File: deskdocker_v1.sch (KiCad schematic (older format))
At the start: 117 parts, among them J1 USB_C_Receptacle_USB2.0, J2 USB_C_Receptacle_USB2.0, J3 OLED, SW1 SW_PUSH, SW10 SW_PUSH, SW11 SW_PUSH, SW12 SW_PUSH, SW13 SW_PUSH, SW14 SW_PUSH, SW15 SW_PUSH, SW16 SW_PUSH, SW17 SW_PUSH, SW18 SW_PUSH, SW19 Rotary_Encoder, SW2 SW_PUSH, SW20 SW_PUSH, SW21 SW_PUSH, SW22 SW_PUSH, SW23 SW_PUSH, SW24 SW_PUSH, SW3 SW_PUSH, SW4 SW_PUSH, SW5 SW_PUSH, SW6 SW_PUSH, SW7 SW_PUSH, SW8 SW_PUSH, SW9 SW_PUSH, U1 ATMEGA32U4, U2 MIC5219-5.0YMM, X1 16Mhz

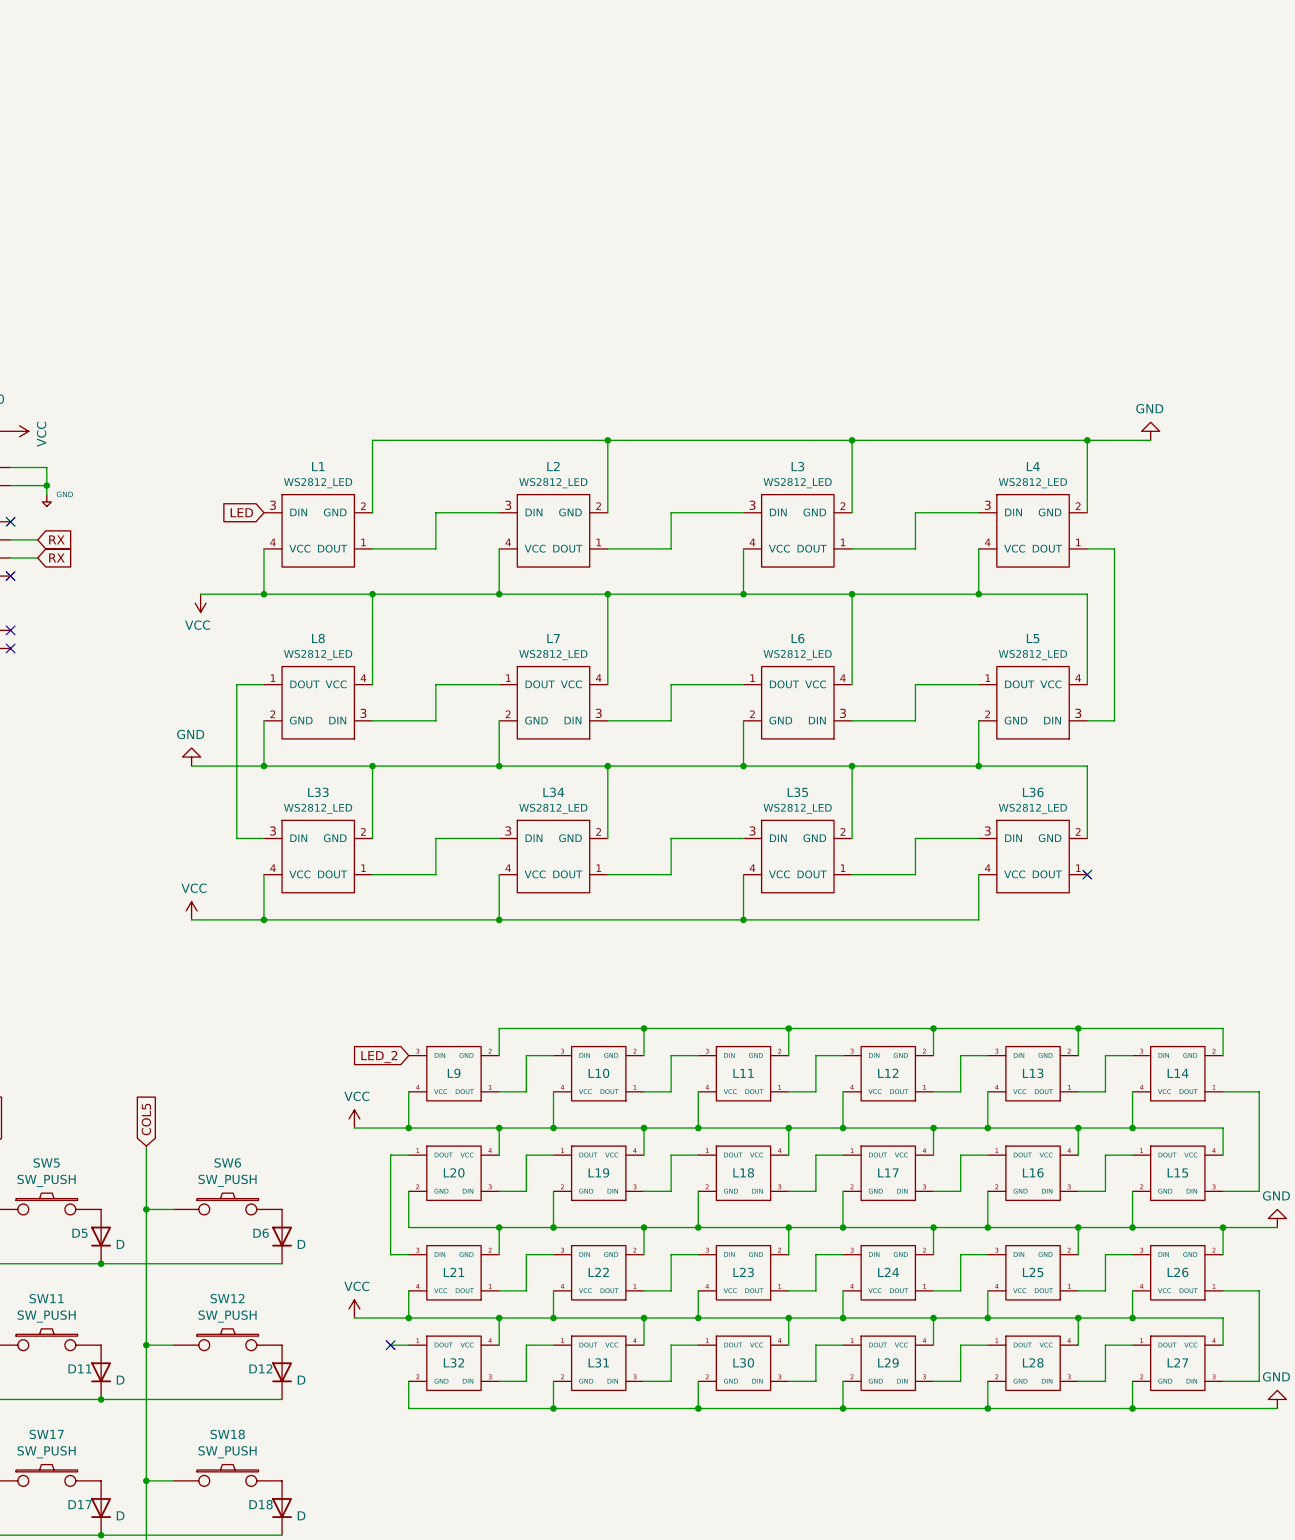
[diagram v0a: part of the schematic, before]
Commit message: schematic final_4
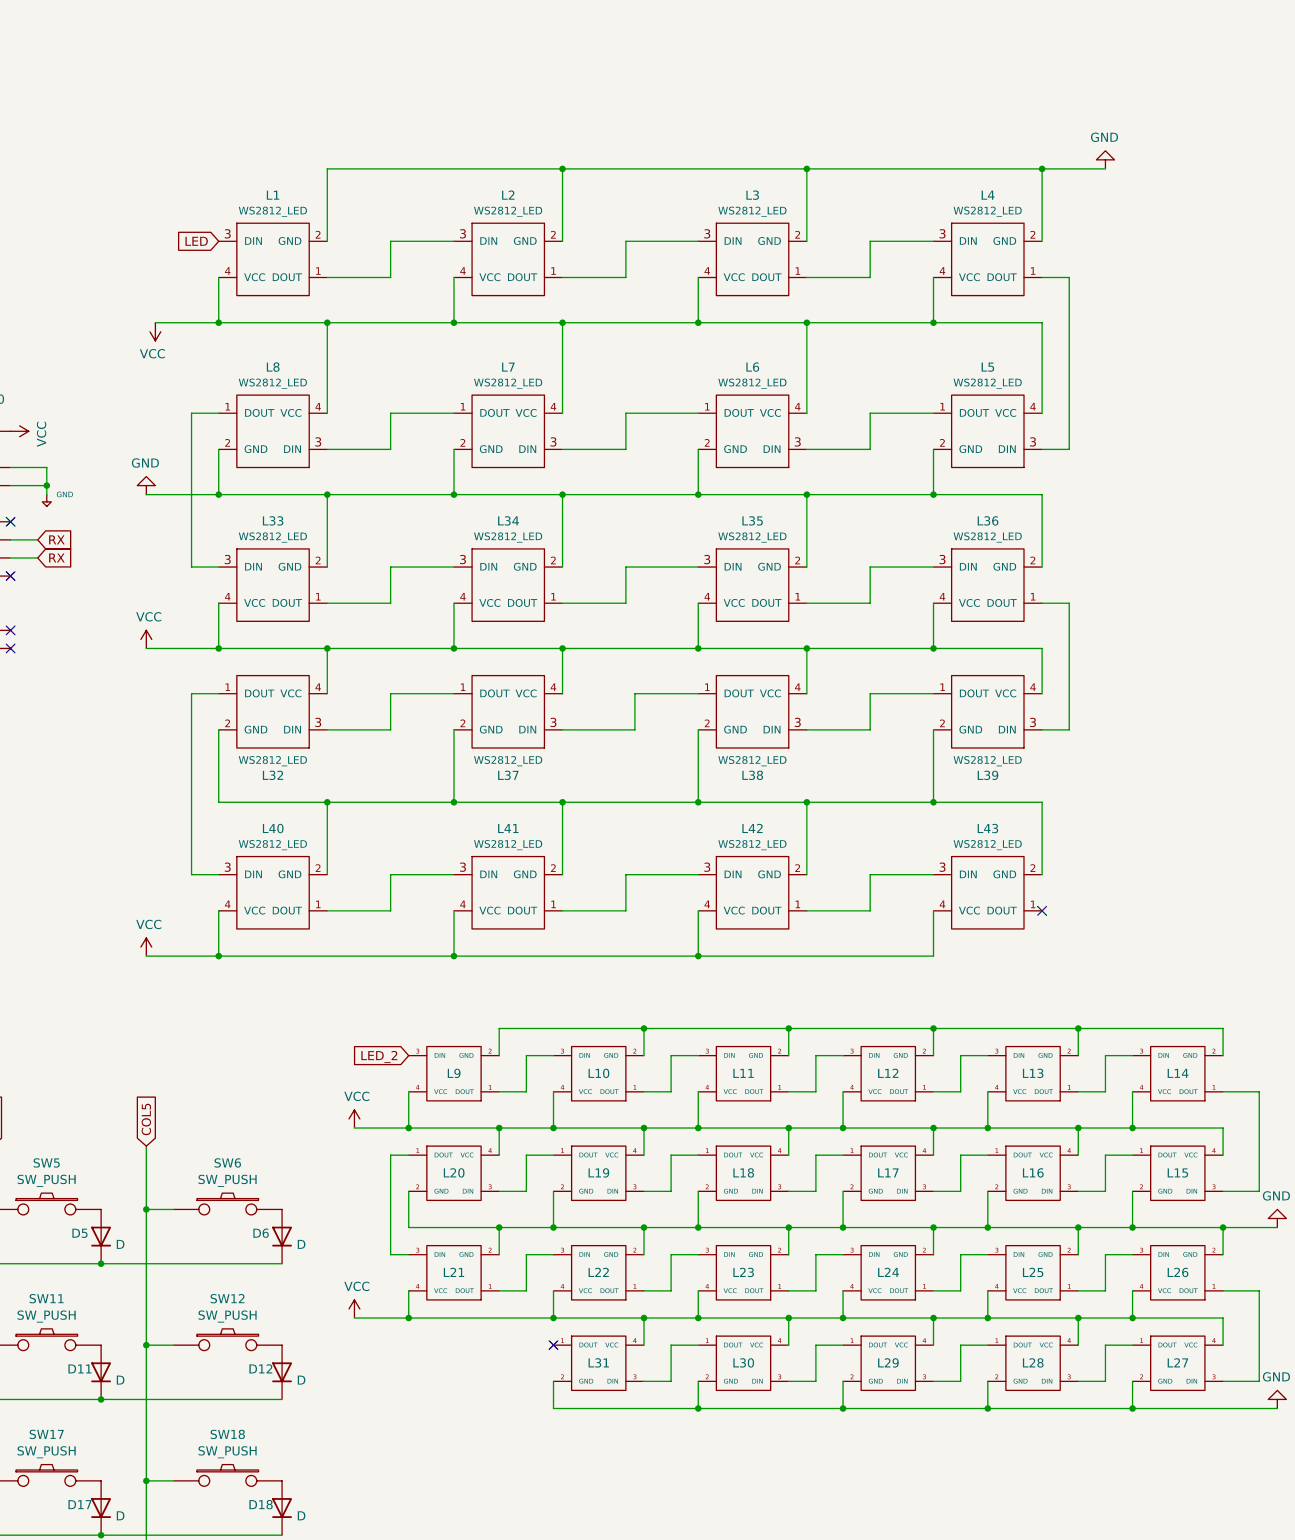
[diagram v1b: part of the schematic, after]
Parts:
- removed L32: SK6812_mini, keebio_parts:SK6812-MINI-E, symbol keyboard_parts:SK6812_mini
- added L32, L37, L38, L39, L40, L41, L42, L43: WS2812_LED, keebio_parts:WS2812B, symbol keyboard_parts:WS2812_LED
- BZ1: footprint Buzzer_Beeper:MagneticBuzzer_PUI_AT-0927-TT-6-R -> reversible-kicad-footprints:Piezo-KLJ-1625
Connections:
- net VCC: now also L32.4 (VCC), L37.4 (VCC), L38.4 (VCC), L39.4 (VCC), L40.4 (VCC), L41.4 (VCC), L42.4 (VCC), L43.4 (VCC)
- net at L36.1 (DOUT): now also L39.3 (DIN)
- new net: L38.3 (DIN), L39.1 (DOUT)
- new net: L32.2 (GND), L37.2 (GND), L38.2 (GND), L39.2 (GND), L40.2 (GND), L41.2 (GND), L42.2 (GND), L43.2 (GND)
- new net: L37.3 (DIN), L38.1 (DOUT)
- new net: L32.3 (DIN), L37.1 (DOUT)
- new net: L32.1 (DOUT), L40.3 (DIN)
- new net: L40.1 (DOUT), L41.3 (DIN)
- new net: L41.1 (DOUT), L42.3 (DIN)
- new net: L42.1 (DOUT), L43.3 (DIN)
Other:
- moved on the sheet: L1, L2, L3, L33, L34, L35, L36, L4, L5, L6, L7, L8
